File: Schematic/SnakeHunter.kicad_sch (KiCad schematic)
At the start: 17 parts, among them J1 Conn_01x04_Pin, J2 Conn_01x04_Pin, SW1 SW_Nidec_CAS-120A1, SW3 SW_DIP_x02, U2 CR2013-MI2120, U3 TSDP341xx, U4 NRF24L01_Breakout, U5 CRE1S0305S3C

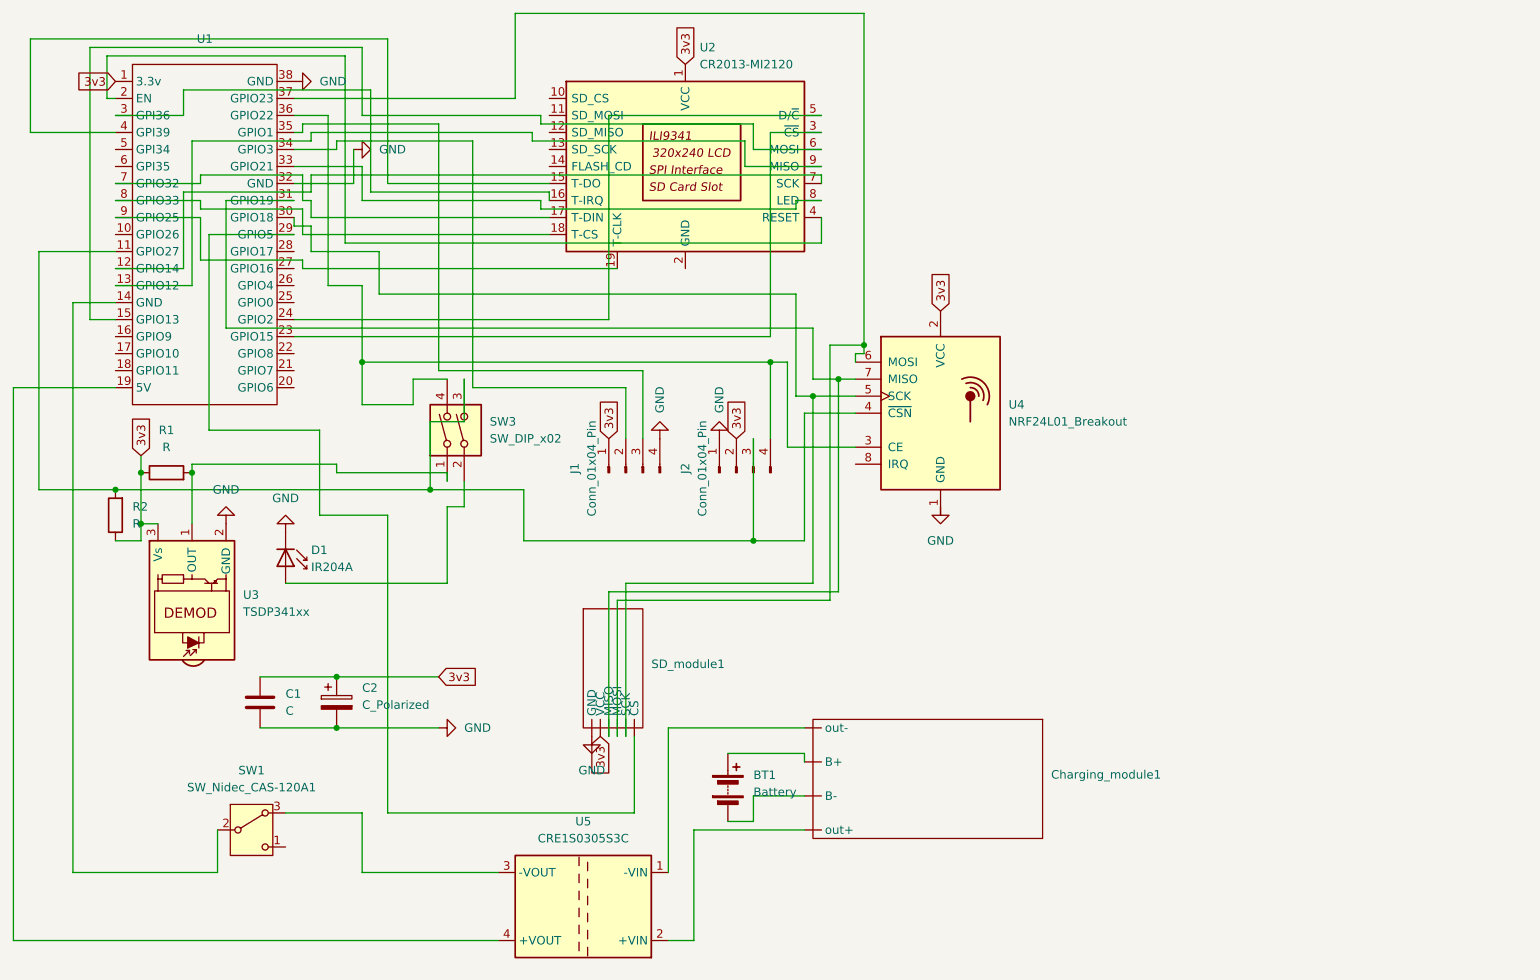
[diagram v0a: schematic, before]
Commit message: Schematic moreee cleannn
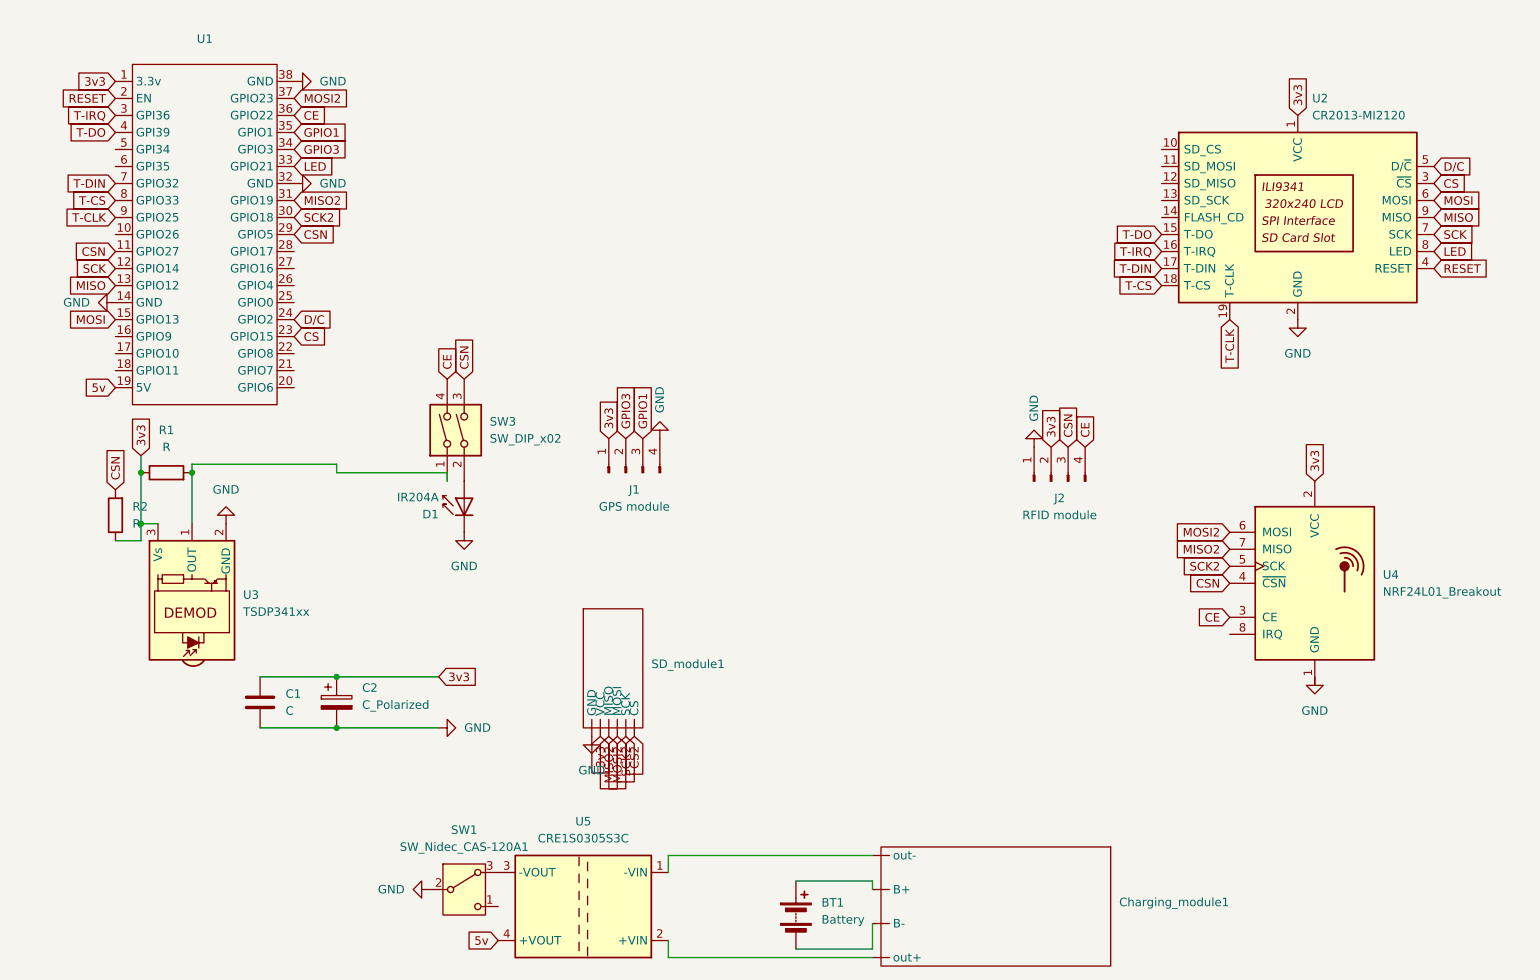
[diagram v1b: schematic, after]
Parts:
- J1: value Conn_01x04_Pin -> GPS module
- J2: value Conn_01x04_Pin -> RFID module
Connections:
- net GND: now also SW1.2 (B), U1.14 (GND), U2.2 (GND)
- net T-DO: now reaches U1.4 (GPI39), U2.15 (T-DO)
- net T-IRQ: now reaches U1.3 (GPI36), U2.16 (T-IRQ)
- net T-DIN: now reaches U1.7 (GPIO32), U2.17 (T-DIN)
- net T-CS: now reaches U1.8 (GPIO33), U2.18 (T-CS)
- net T-CLK: now reaches U1.9 (GPIO25), U2.19 (T-CLK)
- net CS: now reaches U1.23 (GPIO15), U2.3 (~{CS})
- net RESET: now reaches U1.2 (EN), U2.4 (RESET)
- net D/C: now reaches U1.24 (GPIO2), U2.5 (D/~{C})
- net MOSI: now reaches U1.15 (GPIO13), U2.6 (MOSI)
- net SCK: now reaches U1.12 (GPIO14), U2.7 (SCK)
- net LED: now reaches U1.33 (GPIO21), U2.8 (LED)
- net MISO: now reaches U1.13 (GPIO12), U2.9 (MISO)
- net CSN: now reaches U1.29 (GPIO5)
- net CSN: now also J2.3 (Pin_3), R2.2, SW3.3, U1.11 (GPIO27), U4.4 (~{CSN}); no longer SD_module1. (CS)
- net SCK2: now reaches SD_module1. (CS), U1.30 (GPIO18), U4.5 (SCK)
- net MISO2: now reaches SD_module1. (CS), U1.31 (GPIO19), U4.7 (MISO)
- net MOSI2: now reaches SD_module1. (CS), U1.37 (GPIO23), U4.6 (MOSI)
- net CE: now reaches J2.4 (Pin_4), SW3.4, U1.36 (GPIO22), U4.3 (CE)
- net 5v: now reaches U1.19 (5V), U5.4 (+VOUT)
- net GPIO3: now reaches J1.2 (Pin_2), U1.34 (GPIO3)
- net GPIO1: now reaches J1.3 (Pin_3), U1.35 (GPIO1)
- new net CS2: SD_module1. (CS)
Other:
- moved on the sheet: BT1, Charging_module1, D1, J2, SW1, U2, U4
